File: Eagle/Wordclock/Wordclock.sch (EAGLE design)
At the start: 79 parts, among them IC1 74HC595D, IC2 74HC595D, IC3 74HC595D, IC4 74HC595D, IC5 74HC595D, IC6 74HC595D, IC7 74HC595D, IC8 74HC595D

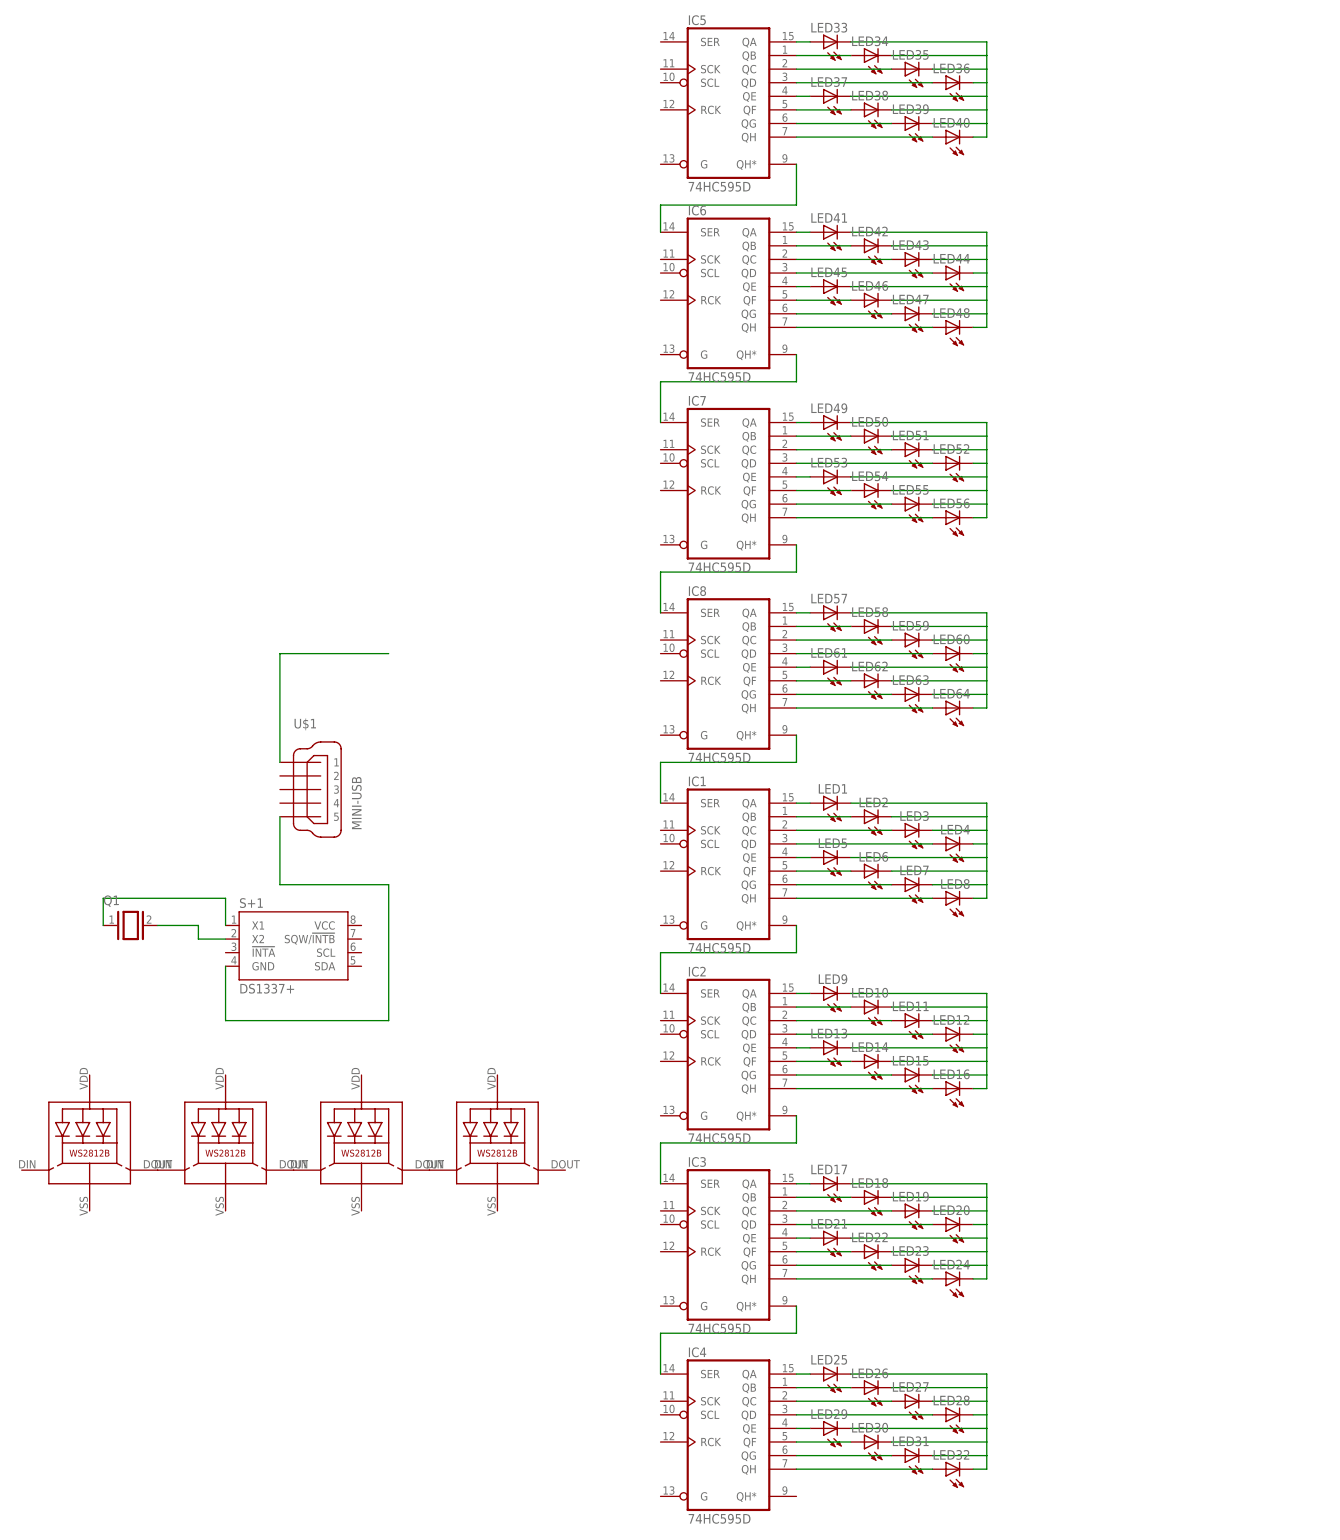
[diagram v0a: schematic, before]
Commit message: Eagle Fehler verbessert
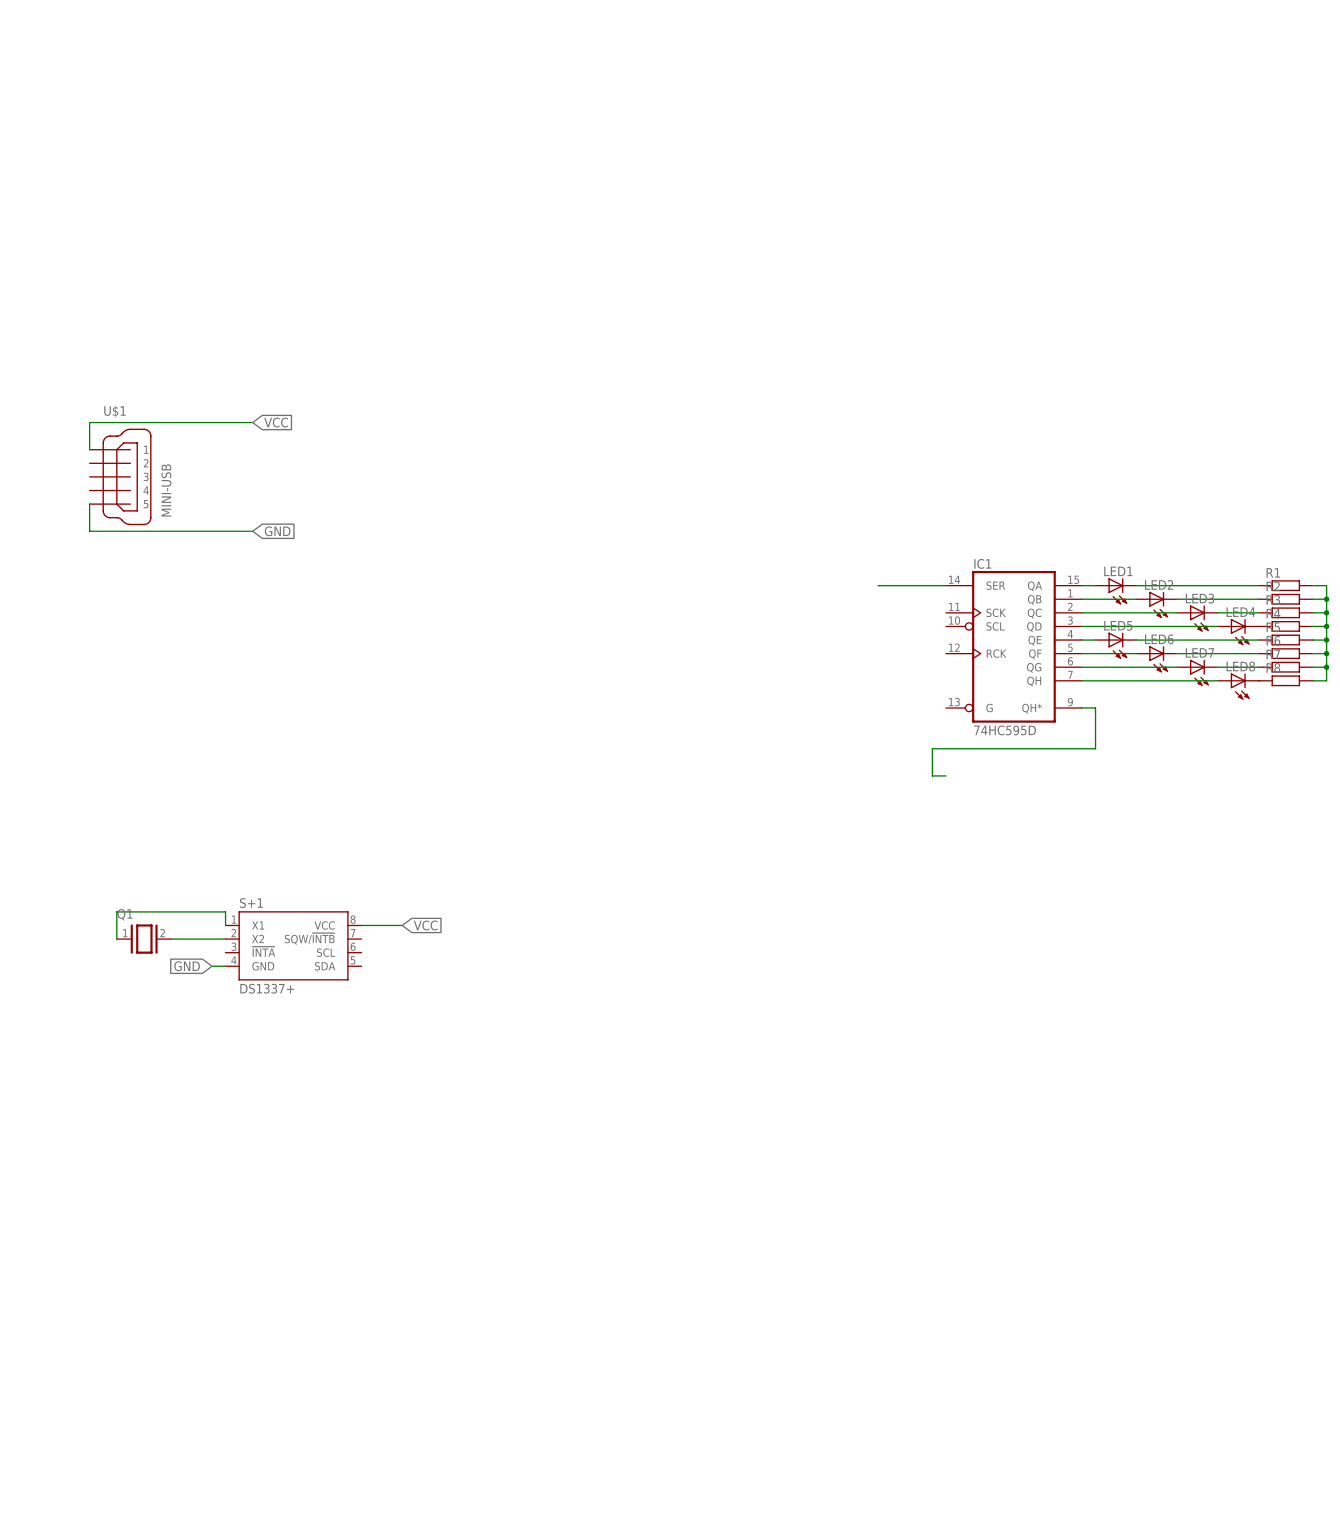
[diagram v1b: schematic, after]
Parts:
- removed IC2, IC3, IC4, IC5, IC6, IC7, IC8: 74HC595D, 74xx-eu:74HC595D
- removed LED10, LED11, LED12, LED13, LED14, LED15, LED16, LED17, LED18, LED19, LED20, LED21, LED22, LED23, LED24, LED25, LED26, LED27, LED28, LED29, LED30, LED31, LED32, LED33, LED34, LED35, LED36, LED37, LED38, LED39, LED40, LED41, LED42, LED43, LED44, LED45, LED46, LED47, LED48, LED49, LED50, LED51, LED52, LED53, LED54, LED55, LED56, LED57, LED58, LED59, LED60, LED61, LED62, LED63, LED64, LED9: (no value), led:LED3MM
- removed LED65, LED66, LED67, LED68: WS2812B, WS2812B:WS2812B
- added R1, R2, R3, R4, R5, R6, R7, R8: (no value), resistor:R-EU_MELF0102W
- LED1, LED2, LED3, LED4, LED5, LED6, LED7, LED8: device led:LED3MM -> led:LED
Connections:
- net N$81 renamed GND
- removed net N$20 (its old number): IC3A.QB, LED18.A
- removed net N$21 (its old number): IC3A.QC, LED19.A
- removed net N$22: IC3A.QE, LED21.A
- removed net N$23: IC3A.QD, LED20.A
- removed net N$24: IC3A.QF, LED22.A
- removed net N$25: IC3A.QG, LED23.A
- removed net N$26: IC3A.QH, LED24.A
- removed net N$27: LED17.C, LED18.C, LED19.C, LED20.C, LED21.C, LED22.C, LED23.C, LED24.C
- removed net N$28: IC4A.QA, LED25.A
- removed net N$29: IC4A.QB, LED26.A
- removed net N$30: IC4A.QC, LED27.A
- removed net N$31: IC4A.QE, LED29.A
- removed net N$32: IC4A.QD, LED28.A
- removed net N$33: IC4A.QF, LED30.A
- removed net N$34: IC4A.QG, LED31.A
- removed net N$35: IC4A.QH, LED32.A
- removed net N$36: LED25.C, LED26.C, LED27.C, LED28.C, LED29.C, LED30.C, LED31.C, LED32.C
- removed net N$37: IC5A.QA, LED33.A
- removed net N$38: IC5A.QB, LED34.A
- removed net N$39: IC5A.QC, LED35.A
- removed net N$40: IC5A.QE, LED37.A
- removed net N$41: IC5A.QD, LED36.A
- removed net N$42: IC5A.QF, LED38.A
- removed net N$43: IC5A.QG, LED39.A
- removed net N$44: IC5A.QH, LED40.A
- removed net N$45: LED33.C, LED34.C, LED35.C, LED36.C, LED37.C, LED38.C, LED39.C, LED40.C
- removed net N$46: IC6A.QA, LED41.A
- removed net N$47: IC6A.QB, LED42.A
- removed net N$48: IC6A.QC, LED43.A
- removed net N$49: IC6A.QE, LED45.A
- removed net N$50: IC6A.QD, LED44.A
- removed net N$51: IC6A.QF, LED46.A
- removed net N$52: IC6A.QG, LED47.A
- removed net N$53: IC6A.QH, LED48.A
- removed net N$54: LED41.C, LED42.C, LED43.C, LED44.C, LED45.C, LED46.C, LED47.C, LED48.C
- removed net N$55: IC7A.QA, LED49.A
- removed net N$56: IC7A.QB, LED50.A
- removed net N$57: IC7A.QC, LED51.A
- removed net N$58: IC7A.QE, LED53.A
- removed net N$59: IC7A.QD, LED52.A
- removed net N$60: IC7A.QF, LED54.A
- removed net N$61: IC7A.QG, LED55.A
- removed net N$62: IC7A.QH, LED56.A
- removed net N$63: LED49.C, LED50.C, LED51.C, LED52.C, LED53.C, LED54.C, LED55.C, LED56.C
- removed net N$64: IC8A.QA, LED57.A
- removed net N$65: IC8A.QB, LED58.A
- removed net N$66: IC8A.QC, LED59.A
- removed net N$67: IC8A.QE, LED61.A
- removed net N$68: IC8A.QD, LED60.A
- removed net N$69: IC8A.QF, LED62.A
- removed net N$70: IC8A.QG, LED63.A
- removed net N$71: IC8A.QH, LED64.A
- removed net N$72: LED57.C, LED58.C, LED59.C, LED60.C, LED61.C, LED62.C, LED63.C, LED64.C
- removed net N$73: IC5A.QH*, IC6A.SER
- removed net N$74: IC6A.QH*, IC7A.SER
- removed net N$75: IC7A.QH*, IC8A.SER
- removed net N$76: IC1A.SER, IC8A.QH*
- removed net N$77: IC1A.QH*, IC2A.SER
- removed net N$78: IC2A.QH*, IC3A.SER
- removed net N$79: IC3A.QH*, IC4A.SER
- removed net N$80: U$1.1
- removed net N$85: LED65.DO, LED66.DI
- removed net N$86: LED66.DO, LED67.DI
- removed net N$87: LED67.DO, LED68.DI
- new net VCC: S+1.VCC, U$1.1
- net N$10: now also LED8.C, R8.1; no longer IC2A.QA, LED9.A
- net N$11: now also LED1.C, R1.1; no longer IC2A.QB, LED10.A
- net N$12: now also LED2.C, R2.1; no longer IC2A.QC, LED11.A
- net N$13: now also LED3.C, R3.1; no longer IC2A.QE, LED13.A
- net N$14: now also LED5.C, R5.1; no longer IC2A.QD, LED12.A
- net N$15: now also LED6.C, R6.1; no longer IC2A.QF, LED14.A
- net N$16: now also LED7.C, R7.1; no longer IC2A.QG, LED15.A
- net N$17: now also R1.2, R2.2, R3.2, R4.2, R5.2, R6.2, R7.2, R8.2; no longer IC2A.QH, LED16.A
- net N$18: now also IC1A.SER; no longer LED10.C, LED11.C, LED12.C, LED13.C, LED14.C, LED15.C, LED16.C, LED9.C
- net N$19: now also IC1A.QH*; no longer IC3A.QA, LED17.A
- net N$9: now also R4.1; no longer LED1.C, LED2.C, LED3.C, LED5.C, LED6.C, LED7.C, LED8.C
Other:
- moved on the sheet: IC1, LED1, LED2, LED3, LED4, LED5, LED6, LED7, LED8, Q1, U$1
